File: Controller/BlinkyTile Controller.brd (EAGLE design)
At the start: 78 x 30 mm, 27 parts, among them IC1 74LVC1G17DCK, IC2 74LVC1G17DCK, IC3 74LVC1G17DCK, Q1 CRYSTAL_4PAD2520, SW1 SPST_TACT-EVQQ2, SW2 SPST_TACT-EVQQ2, T2 TEST_PAD-7

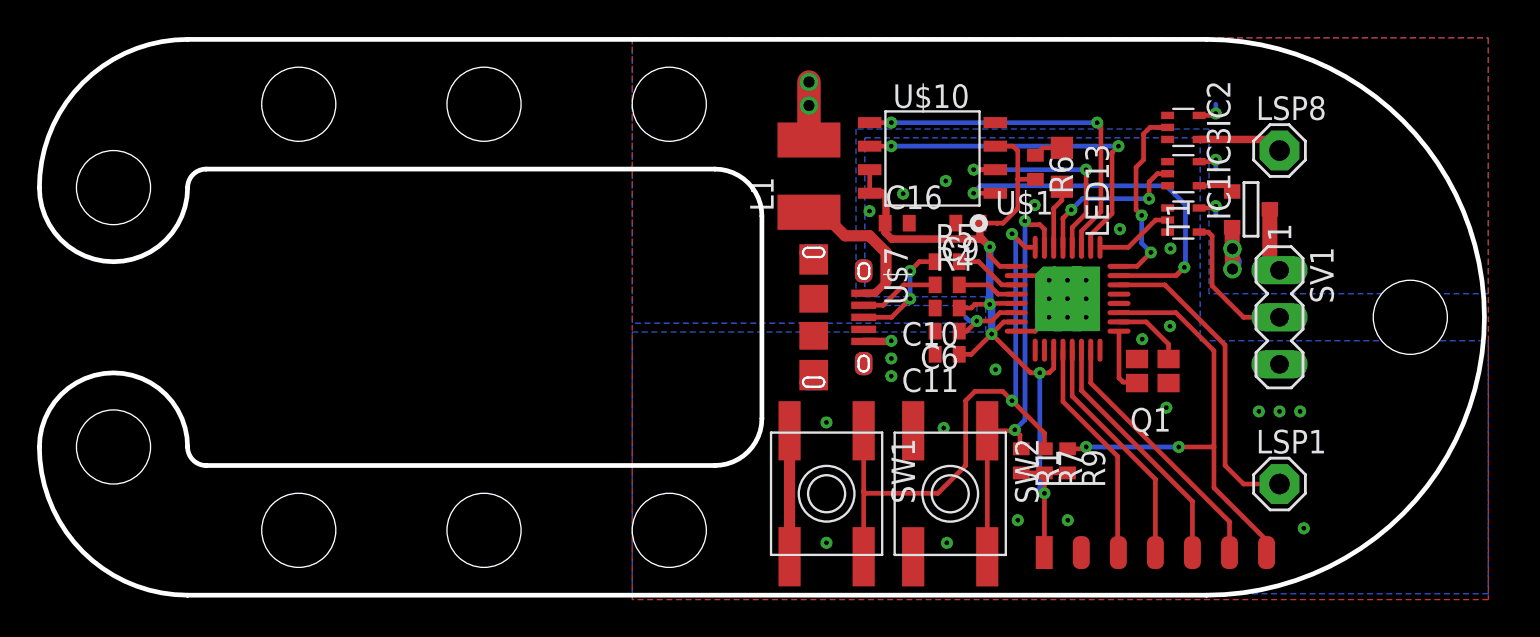
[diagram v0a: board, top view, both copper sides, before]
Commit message: Update to RevB controller from Sam
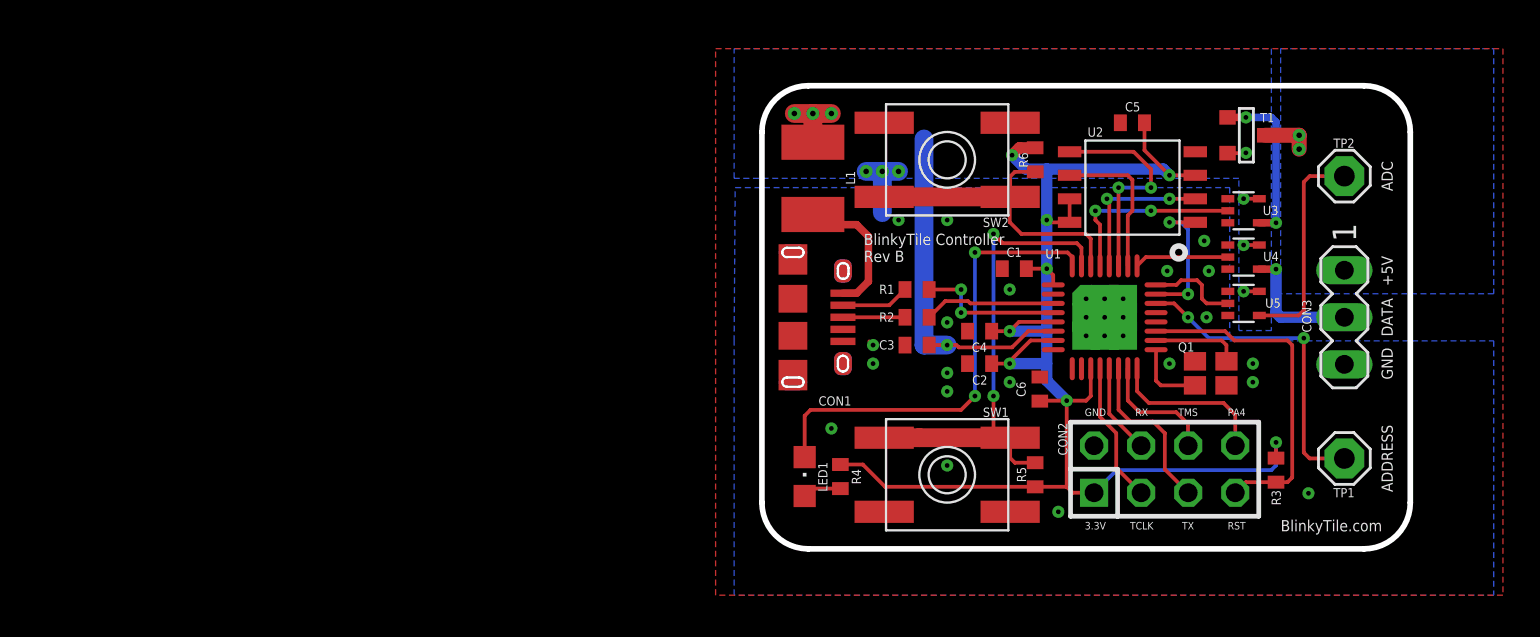
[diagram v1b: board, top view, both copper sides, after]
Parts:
- removed C10: 2.2uF, adafruit:C0402
- removed C11, C16, C9: 100nF, adafruit:C0402
- removed IC1, IC2, IC3: 74LVC1G17DCK, 74xx-little-us:SC70-5
- removed LED13: (no value), adafruit:CHIPLED_0805
- removed LSP1, LSP8: SE11, solpad:SE11
- removed R7: 10k, adafruit:R0402
- removed R9: 1k, adafruit:R0402
- removed SV1: (no value), con-lstb:MA03-1
- removed T2: TEST_PAD-7, Sam Library:TEST_PAD-7
- removed U$1: MK20D--VFM5, blinkinlabs:QFN32_5X5_LONGLEADS
- removed U$10: W25Q80BV, Blinkin_Labs:SOIC8
- removed U$7: USB_MICROSMT+THRUHULE, blinkinlabs:USB_MICRO_THRUHOLE
- added C1, C2, C3, C5: 100nF, adafruit:C0402
- added C4: 2.2uF, adafruit:C0402
- added CON1: USB_MICROSMT+THRUHULE, blinkinlabs:USB_MICRO_THRUHOLE
- added CON2: F-2X04-DIL-100, con-headers-jp:DIL-100-2X04
- added CON3: (no value), con-lstb:MA03-1
- added LED1: STATUS, adafruit:CHIPLED_0805
- added R2: 33, adafruit:R0402
- added R3: 1k, adafruit:R0402
- added TP1: ADCIN, solpad:SE11
- added TP2: ADDRESS, solpad:SE11
- added U1: MK20D--VFM5, blinkinlabs:QFN32_5X5_LONGLEADS
- added U2: W25Q80BV, Blinkin_Labs:SOIC8
- added U3, U4, U5: 74LVC1G17DCK, 74xx-little-us:SC70-5
- R1: value 10k -> 33
- R4: value 33 -> 1k
- R5: value 33 -> 10k
- R6: value 1k -> 10k
- moved SW2 18.0 mm to (10.0, 8.50), turned to 180 degrees
- moved R5 12.4 mm to (14.8, -8.50), turned to 270 degrees
- moved R4 11.8 mm to (4.24, -8.60), turned to 90 degrees
- moved R1 10.8 mm to (8.38, 1.50), turned to 0 degrees
- moved SW1 6.59 mm to (10.0, -8.50), turned to 0 degrees
- moved C6 5.90 mm to (15.0, -3.88), turned to 90 degrees
- moved T1 4.01 mm to (26.1, 9.80)
- moved Q1 3.13 mm to (24.2, -3.02)
- moved R6 0.40 mm to (14.8, 8.50), turned to 90 degrees
- moved L1 0.24 mm to (2.75, 7.50)
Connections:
- new net PA4: CON2.8, U1.16
- net +3V3: now also C1.1, C2.1, C4.1, C5.1, C6.1, CON2.1, R3.2, R4.2, R5.2, U1.1, U1.11, U1.5, U1.7, U2.3, U2.7, U2.8; no longer C10.1, C11.1, C16.1, C9.1, R1.2, R7.2, R9.2, T2.1, U$1.1, U$1.11, U$1.5, U$1.7, U$10.3, U$10.7, U$10.8
- net +5V: now also C3.1, U1.6, U3.5, U4.5, U5.5; no longer C6.1, IC1.5, IC2.5, IC3.5, U$1.6
- net ADC15: now also TP1.MP, U1.22; no longer LSP1.MP, U$1.22
- net ADDRESS_PROGRAM: now also U1.24, U5.2; no longer IC2.2, U$1.24
- net DATA_OUT: now also U1.25, U4.2; no longer IC1.2, U$1.25
- net FLASH_CS: now also U1.23, U2.1; no longer U$1.23, U$10.1
- net FLASH_MISO: now also U1.28, U2.2; no longer U$1.28, U$10.2
- net FLASH_MOSI: now also U1.27, U2.5; no longer U$1.27, U$10.5
- net FLASH_SCK: now also U1.26, U2.6; no longer U$1.26, U$10.6
- net GND: now also C1.2, C2.2, C3.2, C4.2, C5.2, CON1.PIN$5, CON2.2, CON3.3, U1.2, U1.8, U1.PAD@1, U1.PAD@10, U1.PAD@11, U1.PAD@2, U1.PAD@3, U1.PAD@4, U1.PAD@5, U1.PAD@6, U1.PAD@9, U2.4, U3.3, U4.3, U5.3; no longer C10.2, C11.2, C16.2, C9.2, IC1.3, IC2.3, IC3.3, SV1.3, T2.2, U$1.2, U$1.8, U$1.PAD@1, U$1.PAD@10, U$1.PAD@11, U$1.PAD@2, U$1.PAD@3, U$1.PAD@4, U$1.PAD@5, U$1.PAD@6, U$1.PAD@9, U$10.4, U$7.PIN$5
- net LED_DATA: now also CON3.2, U4.4; no longer IC1.4, SV1.2
- net N$1: now also U1.18; no longer U$1.18
- net N$10: now also CON1.PIN$3, R2.1; no longer R5.1, U$7.PIN$3
- net N$11: now also R1.2, U1.4; no longer R4.2, U$1.4
- net N$12: now also R2.2, U1.3; no longer R5.2, U$1.3
- net N$16: now also LED1.A, R4.1; no longer LED13.A, R6.1
- net N$2: now also U1.17; no longer U$1.17
- net N$3: now also CON1.PIN$1; no longer U$7.PIN$1
- net N$4: now also TP2.MP, U5.4; no longer IC2.4, LSP8.MP
- net N$5: now also CON3.1; no longer SV1.1
- net N$6: now also U3.4; no longer IC3.4
- net N$9: now also CON1.PIN$2, R1.1; no longer R4.1, U$7.PIN$2
- net POWER_ENABLE: now also U1.29, U3.2; no longer IC3.2, U$1.29
- net RESET: now also CON2.7, R3.1, U1.19; no longer R9.1, T2.7, U$1.19
- net RX: now also CON2.4, U1.13; no longer T2.4, U$1.13
- net STATUS: now also LED1.C, U1.32; no longer LED13.C, U$1.30
- net SW1: now also R5.1, U1.31; no longer R7.1, U$1.32
- net SW2: now also R6.1, U1.30; no longer R1.1, U$1.31
- net TCLK: now also CON2.3, U1.12; no longer T2.3, U$1.12
- net TMS: now also CON2.6, U1.15; no longer T2.6, U$1.15
- net TX: now also CON2.5, U1.14; no longer T2.5, U$1.14
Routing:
- net +3V3: track 51.3 -> 80.2 mm, vias 5 -> 8
- net STATUS: track 3.45 -> 25.4 mm, vias 0 -> 2
- net FLASH_CS: track 20.9 -> 7.77 mm
- net +5V: track 14.3 -> 26.6 mm
- net FLASH_SCK: track 19.5 -> 8.24 mm, vias 2 -> 0
- net PA4: track 0.00 -> 8.71 mm
- net GND: track 12.3 -> 4.26 mm
- net RX: track 12.8 -> 4.87 mm
- net FLASH_MOSI: track 19.6 -> 11.8 mm
- net RESET: track 26.0 -> 18.2 mm, vias 2 -> 0
- net TMS: track 14.0 -> 6.67 mm
- net N$4: track 4.59 -> 11.8 mm
- net N$6: track 1.91 -> 9.06 mm, vias 0 -> 2
- net SW2: track 23.8 -> 17.0 mm, vias 2 -> 0
- net SW1: track 33.4 -> 27.1 mm
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- added copper zone on layer 16, net N$5
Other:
- board size 78 x 30 mm -> 35 x 25 mm
- board text added: "+5V"
- board text added: "3.3V"
- board text added: "ADC"
- board text added: "ADDRESS"
- board text added: "BlinkyTile Controller Rev B"
- board text added: "BlinkyTile.com"
- board text added: "DATA"
- board text added: "GND"
- board text added: "PA4"
- board text added: "RST"
- board text added: "RX"
- board text added: "TCLK"
- board text added: "TMS"
- board text added: "TX"
